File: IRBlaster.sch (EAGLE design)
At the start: 12 parts, among them T4 2N3904, T5 2N3904, T6 2N3904

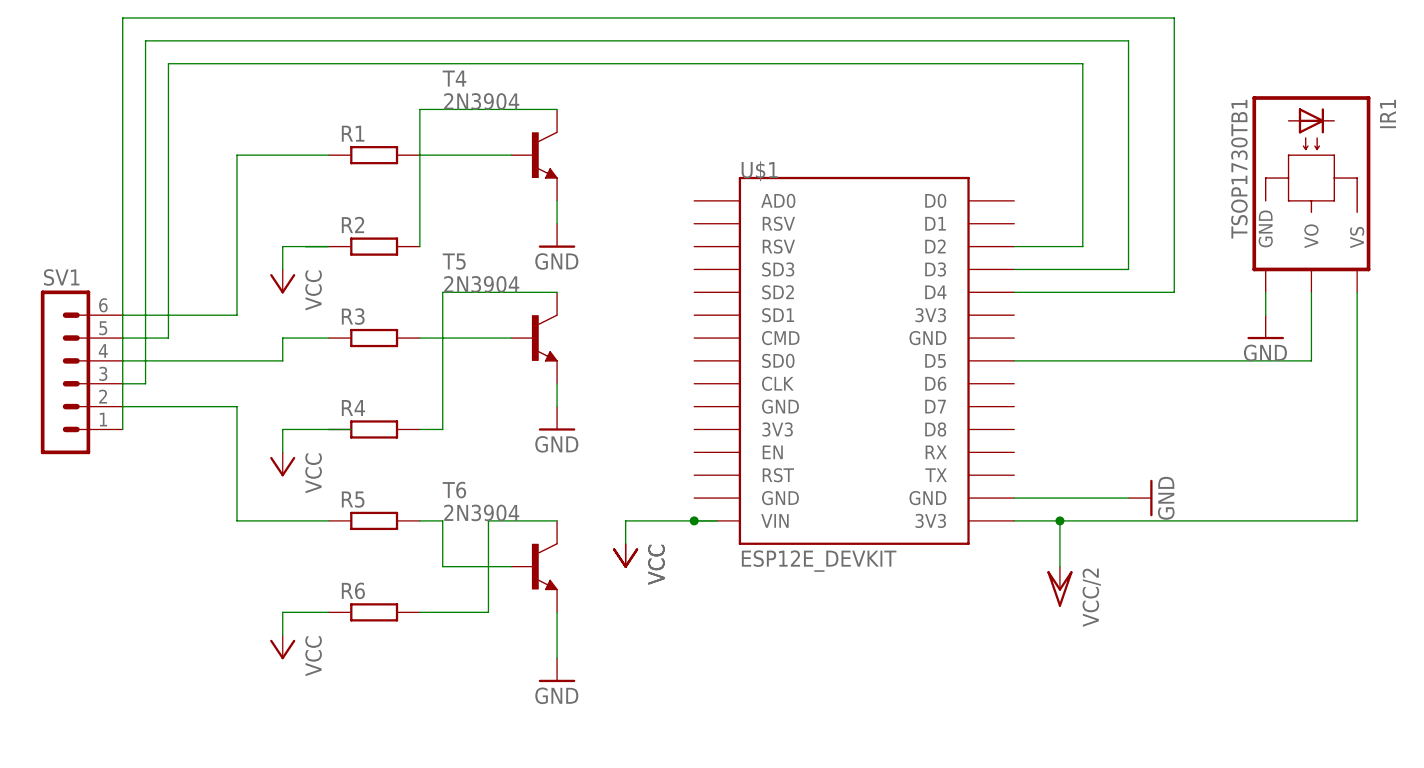
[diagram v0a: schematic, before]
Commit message: Add PCB Files
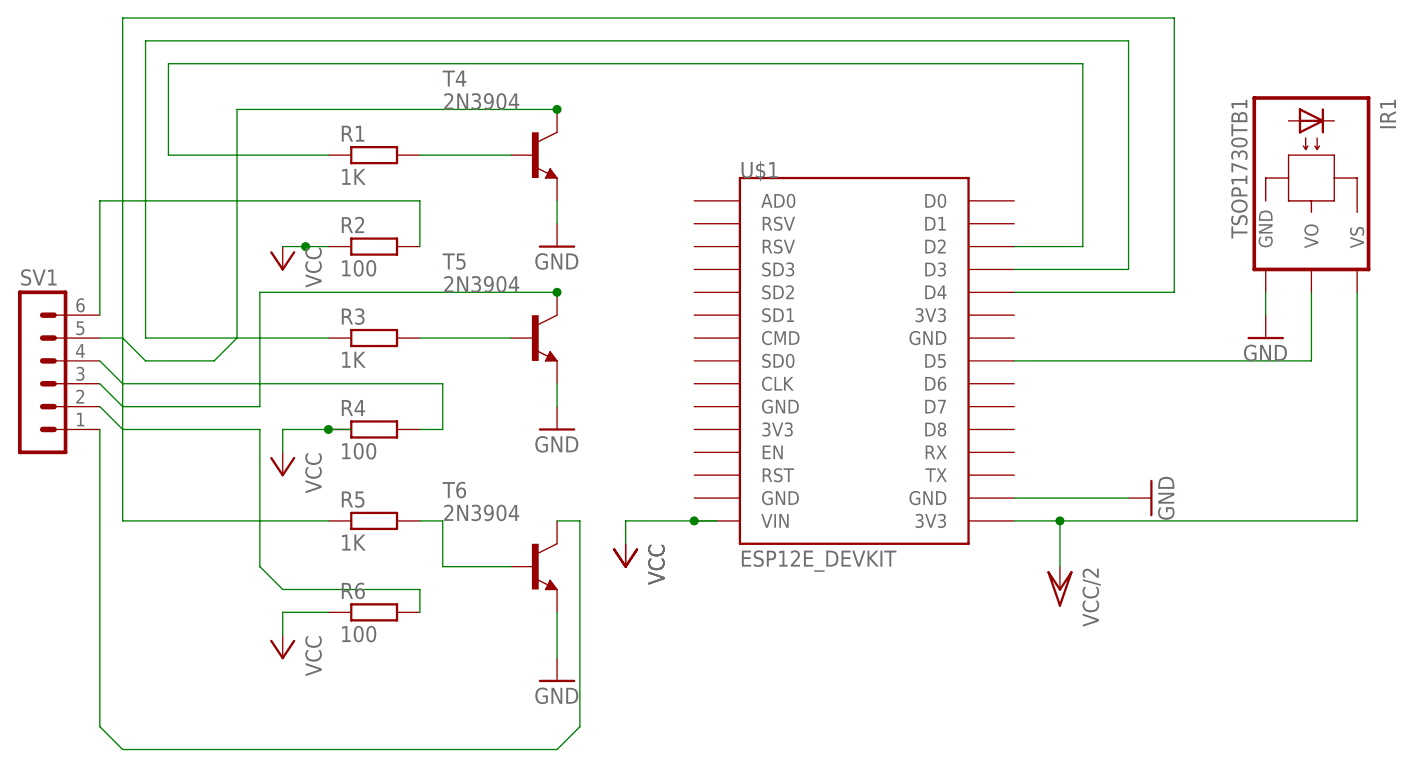
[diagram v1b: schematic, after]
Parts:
- R1, R3, R5: value (none) -> 1K
- R2, R4, R6: value (none) -> 100
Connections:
- removed net N$13: R6.2, T6.C
- removed net N$7: R5.1, SV1.2
- net N$10: now also R3.1; no longer SV1.3
- net N$11: now also SV1.3; no longer R4.2
- net N$12: now also R5.1, R6.2, SV1.2; no longer SV1.1
- net N$14: now also SV1.1, T6.C; no longer R2.1
- net N$5: now also R4.2, SV1.4; no longer R1.1, SV1.6
- net N$6: now also R2.2, SV1.6; no longer R3.1, SV1.4
- net N$8: now also R1.1; no longer SV1.5
- net N$9: now also SV1.5; no longer R2.2
- net VCC: now also R2.1, R4.1
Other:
- moved on the sheet: SV1
